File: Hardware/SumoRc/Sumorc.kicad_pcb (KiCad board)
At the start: 2 copper layers, 50 x 60 mm, 12 parts, among them J1 BTS7960_1, J2 BTS7960_2, SW1 SW_SPDT, U1 ESP32_DevKit_V1_DOIT, U2 LF15_TO220

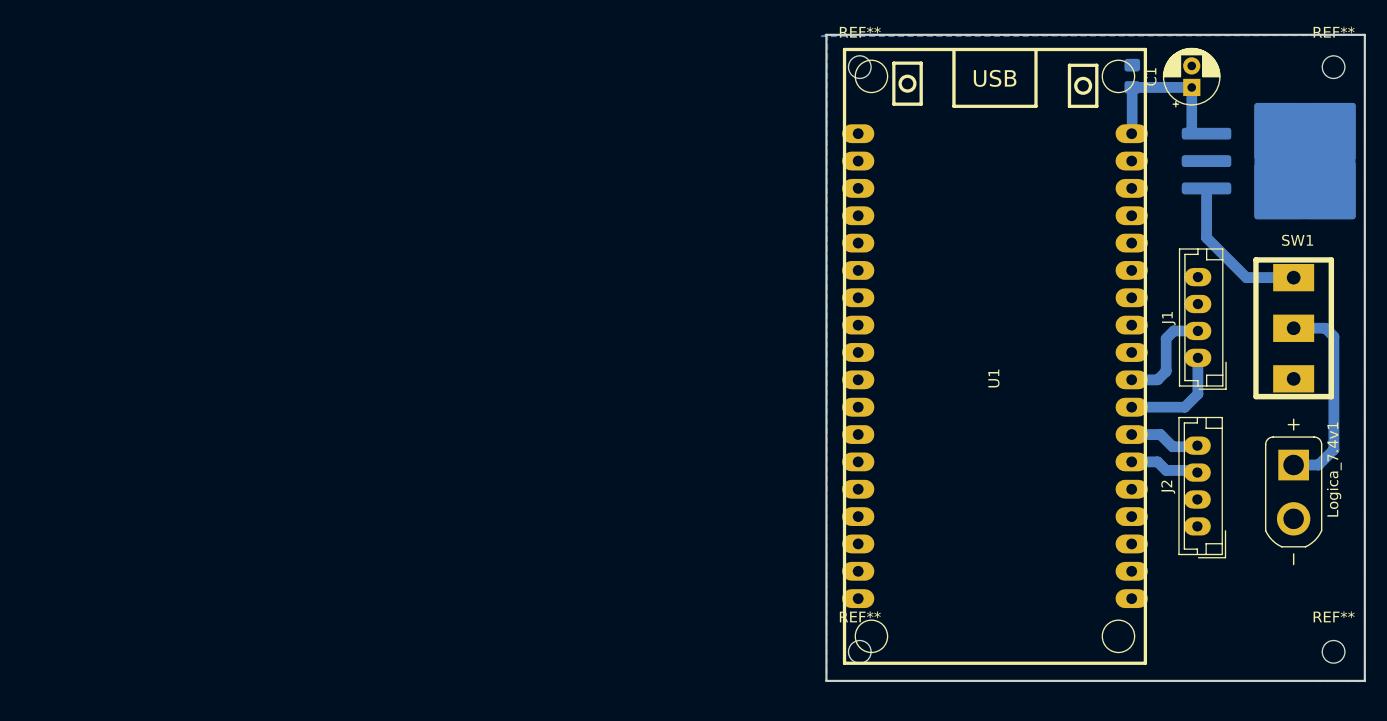
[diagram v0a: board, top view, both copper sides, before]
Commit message: actualizacion
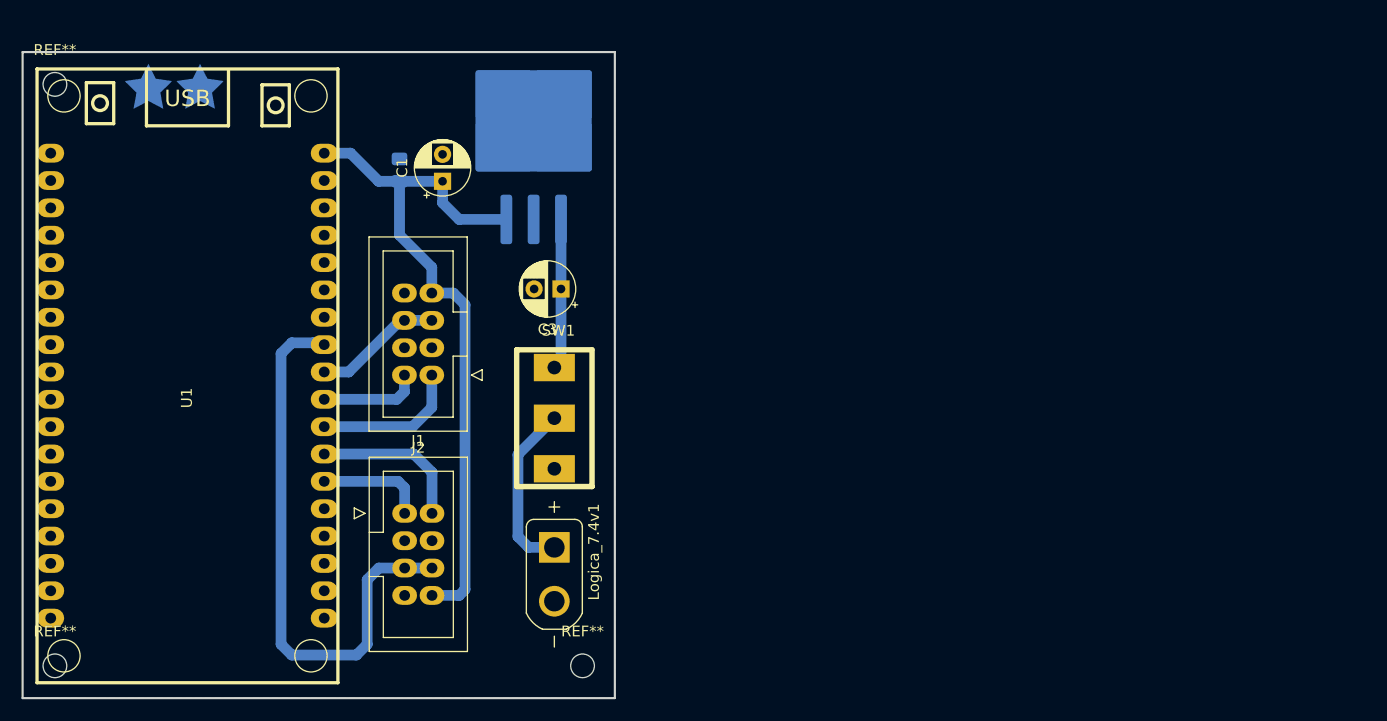
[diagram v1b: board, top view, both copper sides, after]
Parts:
- removed the REF** at (167.8, 48.4)
- removed the REF** at (167.8, 102.7)
- removed the REF** at (123.8, 48.4)
- removed the REF** at (123.8, 102.7)
- added C3: 0.33uF, Capacitor_THT:CP_Radial_D5.0mm_P2.50mm, F.Cu at (96.0, 69.0)
- added G***: LOGO, RamLib:5i, B.Cu at (60.0, 50.0)
- added REF**: MountingHole_2.2mm_M2, MountingHole:MountingHole_2.2mm_M2, F.Cu at (49.0, 104.0)
- added REF**: MountingHole_2.2mm_M2, MountingHole:MountingHole_2.2mm_M2, F.Cu at (98.0, 104.0)
- added REF**: MountingHole_2.2mm_M2, MountingHole:MountingHole_2.2mm_M2, F.Cu at (49.0, 50.0)
- C1: footprint Capacitor_THT:CP_Radial_D5.0mm_P2.00mm -> Capacitor_THT:CP_Radial_D5.0mm_P2.50mm
- J1: value BTS7960_1 -> Screw_Terminal_01x08; footprint Connector_JST:JST_EH_B4B-EH-A_1x04_P2.50mm_Vertical -> Connector_IDC:IDC-Header_2x04_P2.54mm_Vertical
- J2: value BTS7960_2 -> Screw_Terminal_01x08; footprint Connector_JST:JST_EH_B4B-EH-A_1x04_P2.50mm_Vertical -> Connector_IDC:IDC-Header_2x04_P2.54mm_Vertical
- moved U1 75.0 mm to (61.3, 79.2)
- moved J2 73.6 mm to (81.5, 89.8), turned to 0 degrees
- moved J1 71.2 mm to (84.0, 77.0), turned to 180 degrees
- moved U2 70.2 mm to (93.5, 54.9), turned to 90 degrees
- moved C1 70.1 mm to (85.0, 59.0)
- moved SW1 69.2 mm to (95.4, 81.0)
- moved Logica_7.4v1 69.1 mm to (95.4, 95.5)
- moved C2 68.6 mm to (81.0, 58.0)
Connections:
- J1 pad 3: +5V -> unconnected-(J1-Pin_3-Pad3)
- J1 pad 4: GND -> unconnected-(J1-Pin_4-Pad4)
- J2 pad 1: GND -> LPWM_2
- J2 pad 2: +5V -> RPWM_2
- J2 pad 3: LPWM_2 -> unconnected-(J2-Pin_3-Pad3)
- J2 pad 4: RPWM_2 -> unconnected-(J2-Pin_4-Pad4)
- U1 pad 10: unconnected-(U1-IO27-Pad10) -> L_EN1
- U1 pad 11: unconnected-(U1-IO14-Pad11) -> L_EN2
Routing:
- net L_EN2: track 0.00 -> 52.8 mm
- net +5V: track 14.1 -> 65.5 mm
- net L_EN1: track 0.00 -> 12.0 mm
- net RPWM_2: track 6.61 -> 14.5 mm
- net LPWM_2: track 6.51 -> 10.4 mm
- net LPWM_1: track 10.0 -> 13.7 mm
- net Net-(SW1-B): track 18.9 -> 16.2 mm
- net RPWM_1: track 9.99 -> 9.28 mm
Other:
- board size 50 x 60 mm -> 55 x 60 mm
